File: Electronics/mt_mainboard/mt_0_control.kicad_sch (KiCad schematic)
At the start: 4 parts, among them J3 Screw_Terminal_01x02, J4 Conn_01x03_Pin, U1 INA169, U3 DRV8871DDA

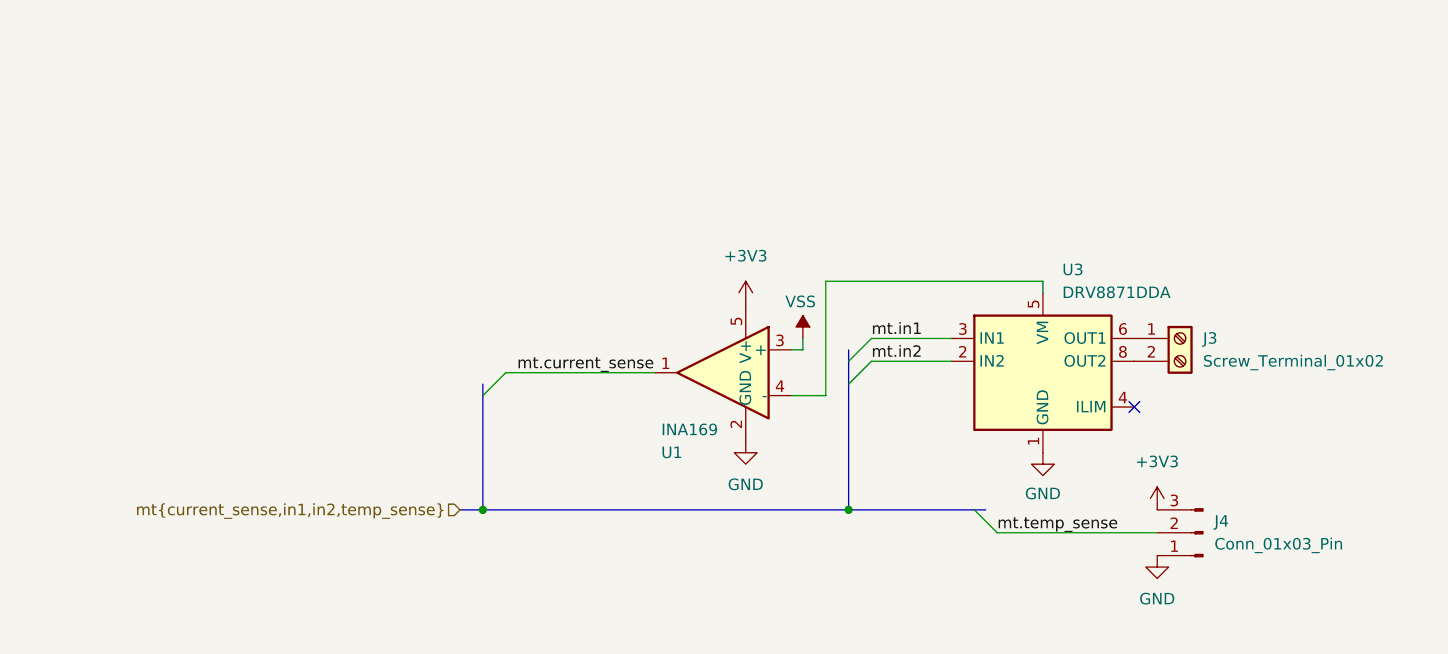
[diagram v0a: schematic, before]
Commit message: backup
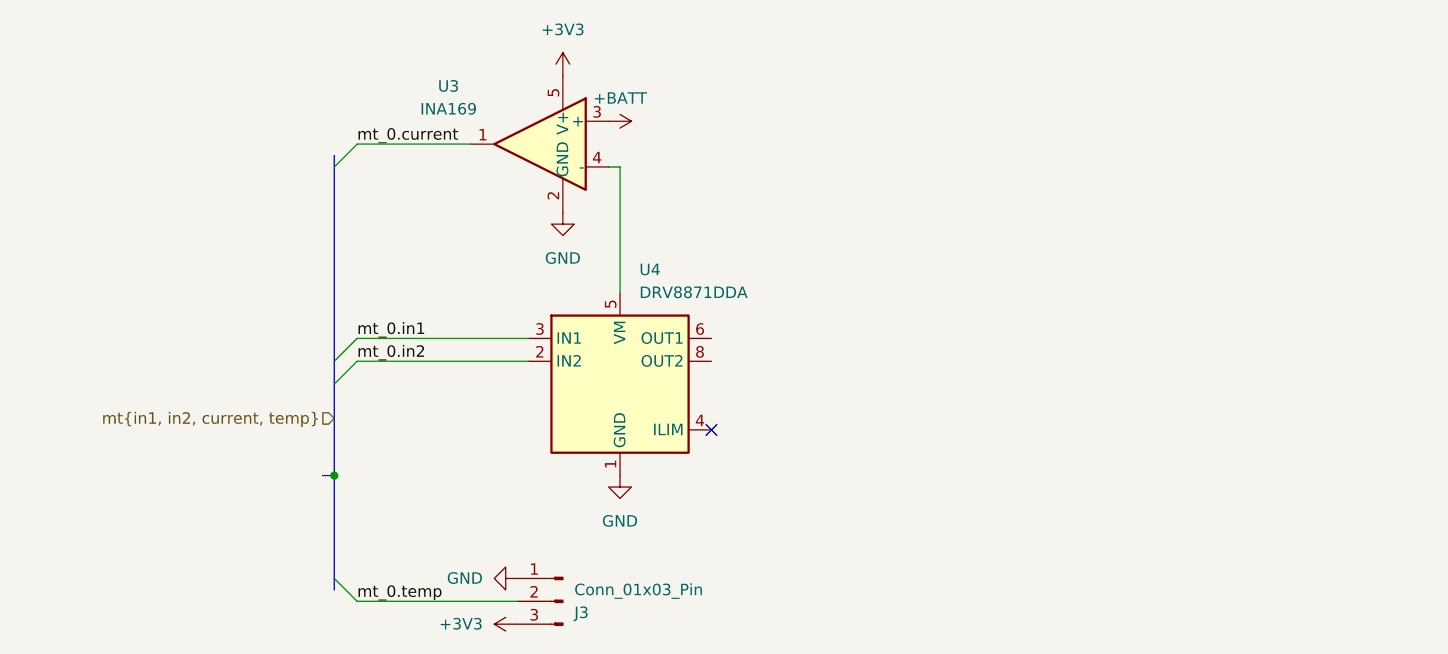
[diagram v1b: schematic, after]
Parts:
- removed J3: Screw_Terminal_01x02, symbol Connector:Screw_Terminal_01x02
- removed J4: Conn_01x03_Pin, symbol Connector:Conn_01x03_Pin
- removed U1: INA169, Package_TO_SOT_SMD:SOT-23-5, symbol Amplifier_Current:INA169
- removed U3: DRV8871DDA, Package_SO:Texas_HTSOP-8-1EP_3.9x4.9mm_P1.27mm_EP2.95x4.9mm_Mask2.4x3.1mm_ThermalVias, symbol Driver_Motor:DRV8871DDA
- added J3: Conn_01x03_Pin, symbol Connector:Conn_01x03_Pin
- added U3: INA169, Package_TO_SOT_SMD:SOT-23-5, symbol Amplifier_Current:INA169
- added U4: DRV8871DDA, Package_SO:Texas_HTSOP-8-1EP_3.9x4.9mm_P1.27mm_EP2.95x4.9mm_Mask2.4x3.1mm_ThermalVias, symbol Driver_Motor:DRV8871DDA
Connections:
- net +3V3: now also J3.3 (Pin_3), U3.5 (V+)
- net GND: now also J3.1 (Pin_1), U3.2 (GND), U4.1 (GND), U4.7 (GND), U4.9 (GND)
- new net: U3.4 (-), U4.5 (VM)
- new net +BATT: U3.3 (+)
- new net mt_0.current: U3.1
- new net mt_0.in1: U4.3 (IN1)
- new net mt_0.in2: U4.2 (IN2)
- new net mt_0.temp: J3.2 (Pin_2)
